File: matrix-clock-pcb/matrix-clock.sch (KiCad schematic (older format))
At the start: 17 parts, among them J1 download, J2 Conn_02x08_Counter_Clockwise, U1 ESP32-WROOM-32D, U2 SHTC3, U3 TXB0108PWR, U4 TXB0108PWR

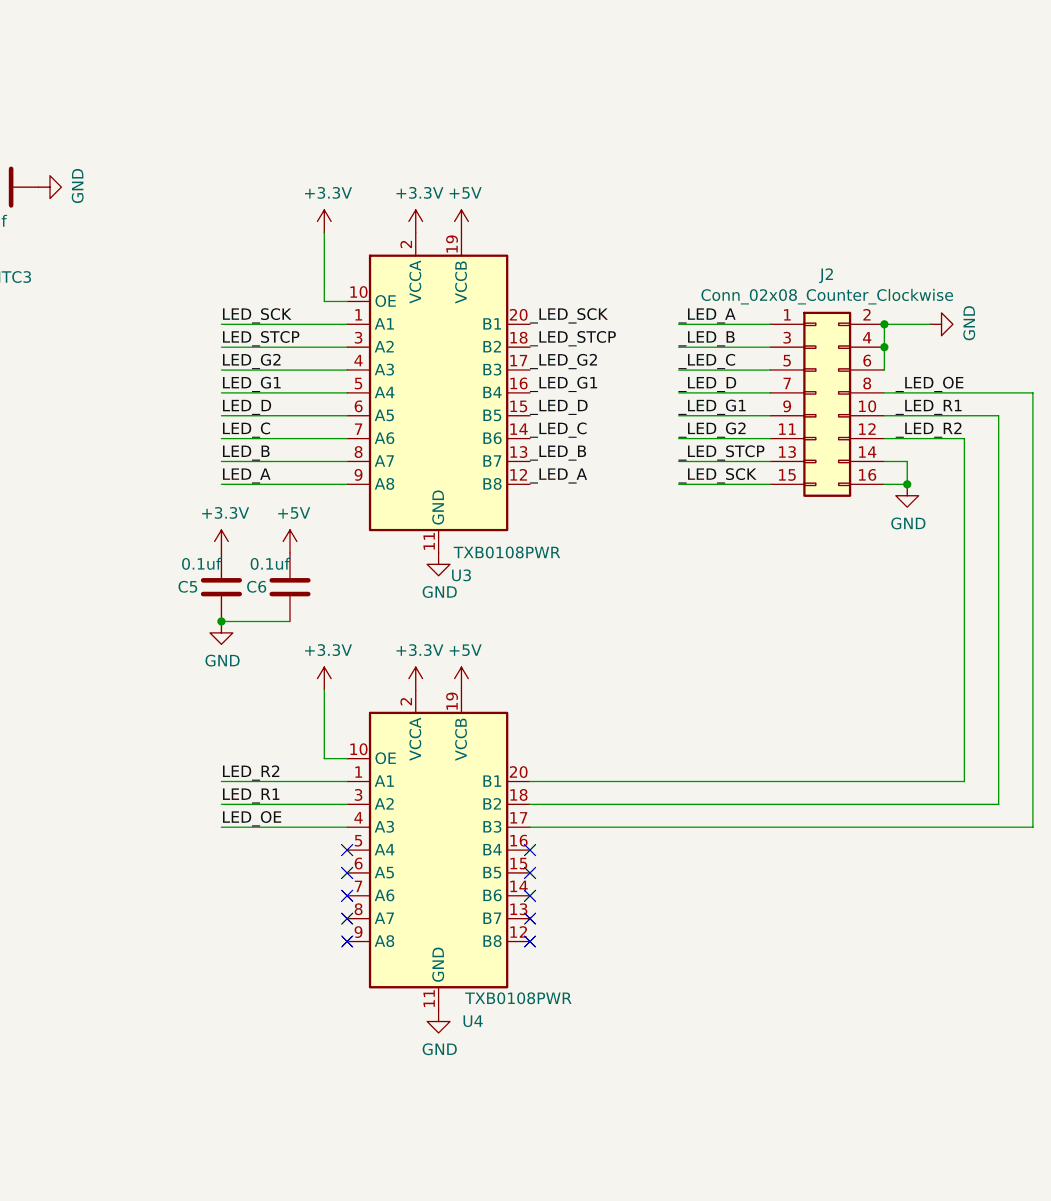
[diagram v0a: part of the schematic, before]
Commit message: pcb: update pcb to v1.1
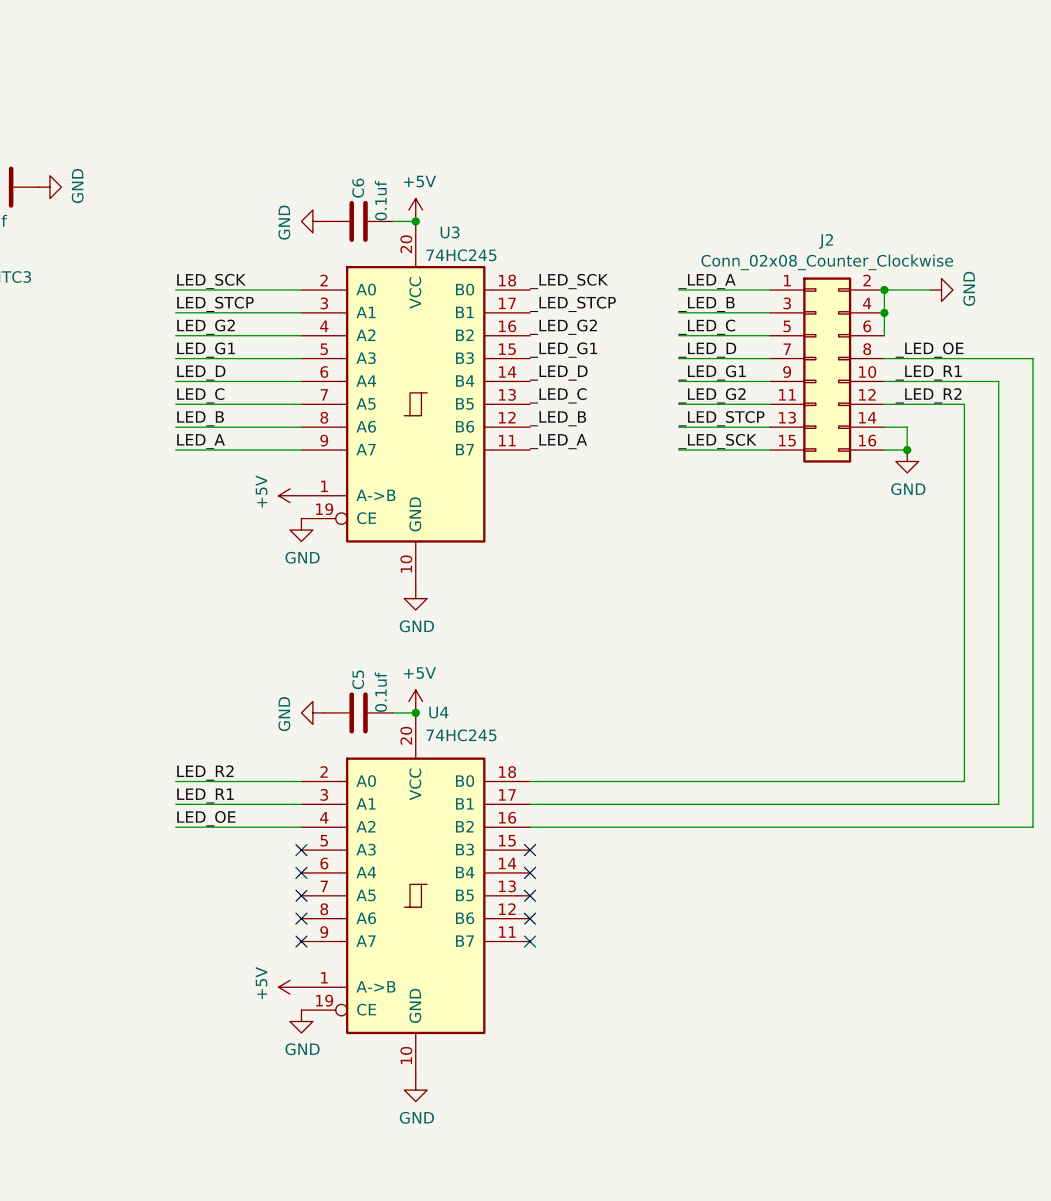
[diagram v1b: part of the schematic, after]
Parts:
- removed U3, U4: TXB0108PWR, Package_SO:TSSOP-20_4.4x6.5mm_P0.65mm, symbol mylib:TXB0108PWR
- added U3, U4: 74HC245, Package_SO:TSSOP-20_4.4x6.5mm_P0.65mm, symbol 74xx:74HC245
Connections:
- net +3V3: no longer C5.2
- net +5V: now also C5.2, U3.1 (A->B), U3.20 (VCC), U4.1 (A->B), U4.20 (VCC)
- net GND: now also U3.10 (GND), U3.19 (CE), U4.10 (GND), U4.19 (CE)
- net LED_A: now also U3.9 (A7)
- net LED_B: now also U3.8 (A6)
- net LED_C: now also U3.7 (A5)
- net LED_D: now also U3.6 (A4)
- net LED_G1: now also U3.5 (A3)
- net LED_G2: now also U3.4 (A2)
- net LED_OE: now also U4.4 (A2)
- net LED_R1: now also U4.3 (A1)
- net LED_R2: now also U4.2 (A0)
- net LED_SCK: now also U3.2 (A0)
- net LED_STCP: now also U3.3 (A1)
- net _LED_A: now also U3.11 (B7)
- net _LED_B: now also U3.12 (B6)
- net _LED_C: now also U3.13 (B5)
- net _LED_D: now also U3.14 (B4)
- net _LED_G1: now also U3.15 (B3)
- net _LED_G2: now also U3.16 (B2)
- net _LED_OE: now also U4.16 (B2)
- net _LED_R1: now also U4.17 (B1)
- net _LED_R2: now also U4.18 (B0)
- net _LED_SCK: now also U3.18 (B0)
- net _LED_STCP: now also U3.17 (B1)
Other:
- moved on the sheet: C5, C6, J2
